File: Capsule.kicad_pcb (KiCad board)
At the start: 2 copper layers, 233.5 x 62.1 mm, 77 parts, among them J1 USB_C_Receptacle_USB2.0, SW1 SW_Push, SW10 SW_Push, SW11 SW_Push, SW12 SW_Push, SW13 SW_Push, SW14 SW_Push, SW15 SW_Push, SW16 SW_Push, SW17 SW_Push, SW18 SW_Push, SW19 SW_Push, SW2 SW_Push, SW20 SW_Push, SW21 SW_Push, SW22 SW_Push, SW23 SW_Push, SW24 SW_Push, SW25 SW_Push, SW26 SW_Push, SW27 SW_Push, SW28 SW_Push, SW29 SW_Push, SW3 SW_Push, SW30 SW_Push, SW4 SW_Push, SW5 SW_Push, SW6 SW_Push, SW7 SW_Push, SW8 SW_Push, SW9 SW_Push, U1 ATmega32U4-A, U2 TPD2S017, Y1 Crystal_GND24

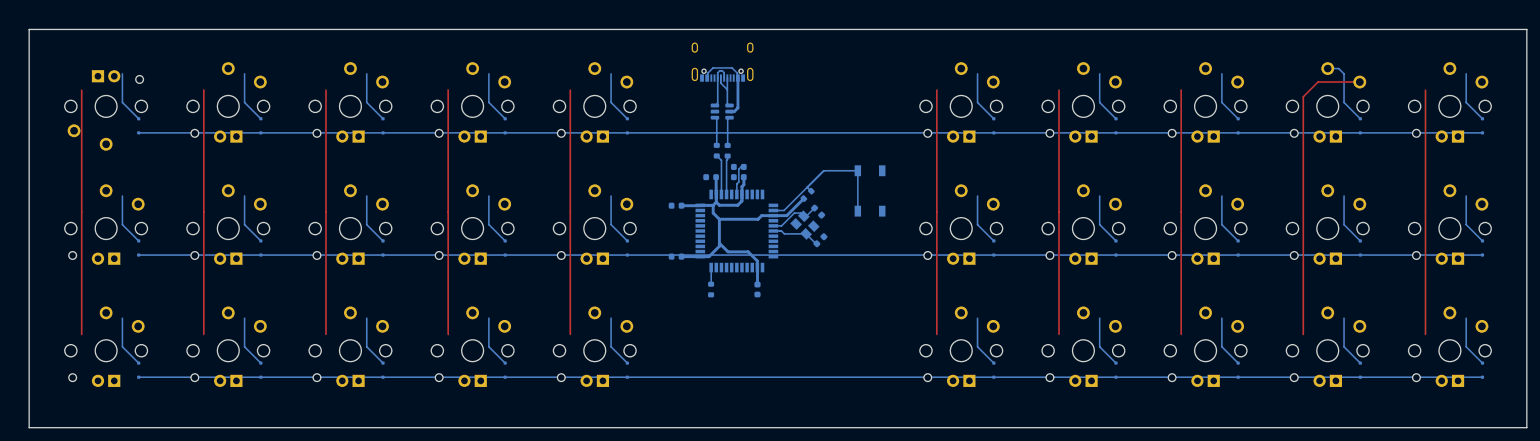
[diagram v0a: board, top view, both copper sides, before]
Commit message: pcb refactor
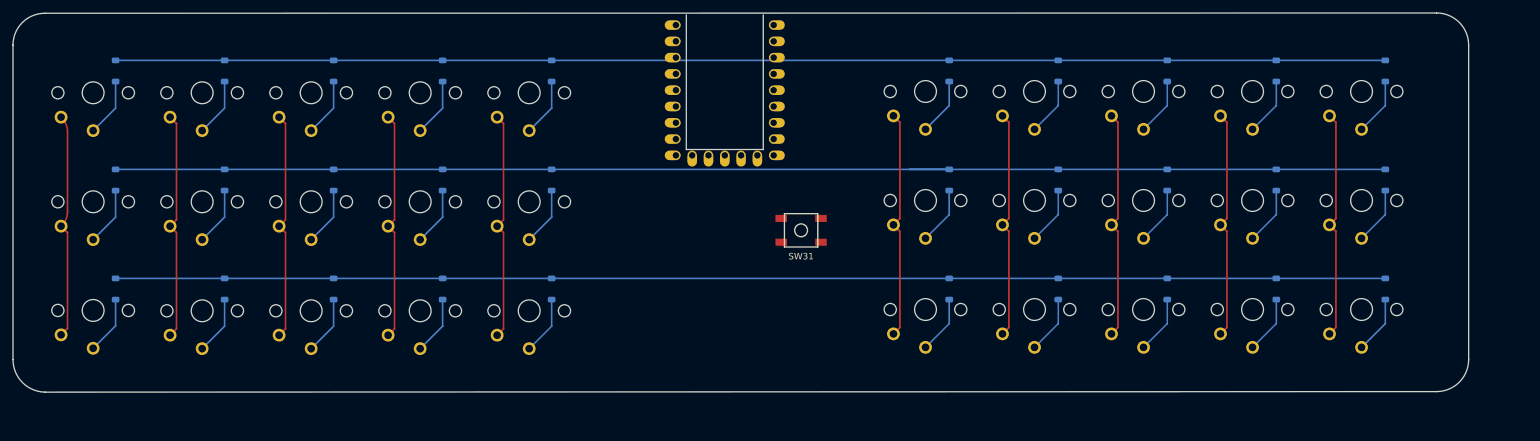
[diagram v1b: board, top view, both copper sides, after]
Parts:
- removed C1, C2: 22p, C_0603_1608Metric
- removed C3, C4, C5, C6: 0.1u, C_0603_1608Metric
- removed C7: 4.7u, C_0603_1608Metric
- removed C8: 1u, C_0603_1608Metric
- removed J1: USB_C_Receptacle_USB2.0, USB_C_Receptacle_XKB_U262-16XN-4BVC11
- removed R1, R2: 22, Resistor_SMD:R_0603_1608Metric
- removed R3, R4: 10k, Resistor_SMD:R_0603_1608Metric
- removed RST: SW_SPST, SW_SPST_TL3342
- removed U2: TPD2S017, SOT-23-6
- removed Y1: Crystal_GND24, Crystal_SMD_3225-4Pin_3.2x2.5mm
- added SW31: SW_Push, random-keyboard-parts:SKQG-1155865, F.Cu at (142.9, 53.9)
- D1, D10, D11, D12, D13, D14, D15, D16, D17, D18, D19, D2, D20, D21, D22, D23, D24, D25, D26, D27, D28, D29, D3, D30, D4, D5, D6, D7, D8, D9: footprint D_SOD-323F -> Diode_SMD:D_SOD-123
- SW1, SW10, SW11, SW12, SW13, SW14, SW15, SW16, SW17, SW18, SW19, SW2, SW20, SW21, SW22, SW23, SW24, SW25, SW26, SW27, SW28, SW29, SW3, SW30, SW4, SW5, SW6, SW7, SW8, SW9: value SW_Push -> SW; footprint Kailh_Choc:KailhChoc-1U -> miketronic_fplib:MB_KailhChoc-1U
- U1: value ATmega32U4-A -> rp2040-zero; footprint TQFP-44_10x10mm_P0.8mm -> mcu:rp2040-zero-tht
- moved U1 22.0 mm to (131.0, 32.0), turned to 180 degrees
- moved D30 19.7 mm to (234.0, 63.0), turned to -90 degrees
- moved D20 18.5 mm to (234.0, 46.0), turned to -90 degrees
- moved D29 18.2 mm to (217.0, 63.0), turned to -90 degrees
- moved D10 17.4 mm to (234.0, 29.0), turned to -90 degrees
- moved D25 17.3 mm to (104.0, 63.0), turned to -90 degrees
- moved D19 16.9 mm to (217.0, 46.0), turned to -90 degrees
- moved D28 16.8 mm to (200.0, 63.0), turned to -90 degrees
- moved D24 16.0 mm to (87.0, 63.0), turned to -90 degrees
- moved D15 15.9 mm to (104.0, 46.0), turned to -90 degrees
- moved D9 15.7 mm to (217.0, 29.0), turned to -90 degrees
- moved D27 15.5 mm to (183.0, 63.0), turned to -90 degrees
- moved D18 15.3 mm to (200.0, 46.0), turned to -90 degrees
- moved SW30 14.9 mm to (229.6, 68.9)
- moved D23 14.8 mm to (70.0, 63.0), turned to -90 degrees
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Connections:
- D1 pad 2: N$1 -> Net-(D1-Pad2)
- D10 pad 2: N$10 -> Net-(D10-Pad2)
- D11 pad 2: N$11 -> Net-(D11-Pad2)
- D12 pad 2: N$12 -> Net-(D12-Pad2)
- D13 pad 2: N$13 -> Net-(D13-Pad2)
- D14 pad 2: N$14 -> Net-(D14-Pad2)
- D15 pad 2: N$15 -> Net-(D15-Pad2)
- D16 pad 2: N$16 -> Net-(D16-Pad2)
- D17 pad 2: N$17 -> Net-(D17-Pad2)
- D18 pad 2: N$18 -> Net-(D18-Pad2)
- D19 pad 2: N$19 -> Net-(D19-Pad2)
- D2 pad 2: N$2 -> Net-(D2-Pad2)
- D20 pad 2: N$20 -> Net-(D20-Pad2)
- D21 pad 2: N$21 -> Net-(D21-Pad2)
- D22 pad 2: N$22 -> Net-(D22-Pad2)
- D23 pad 2: N$23 -> Net-(D23-Pad2)
- D24 pad 2: N$24 -> Net-(D24-Pad2)
- D25 pad 2: N$25 -> Net-(D25-Pad2)
- D26 pad 2: N$26 -> Net-(D26-Pad2)
- D27 pad 2: N$27 -> Net-(D27-Pad2)
- D28 pad 2: N$28 -> Net-(D28-Pad2)
- D29 pad 2: N$29 -> Net-(D29-Pad2)
- D3 pad 2: N$3 -> Net-(D3-Pad2)
- D30 pad 2: N$30 -> Net-(D30-Pad2)
- D4 pad 2: N$4 -> Net-(D4-Pad2)
- D5 pad 2: N$5 -> Net-(D5-Pad2)
- D6 pad 2: N$6 -> Net-(D6-Pad2)
- D7 pad 2: N$7 -> Net-(D7-Pad2)
- D8 pad 2: N$8 -> Net-(D8-Pad2)
- D9 pad 2: N$9 -> Net-(D9-Pad2)
- SW1 pad 1: COL0 -> Net-(D1-Pad2)
- SW1 pad 2: N$1 -> COL0
- SW10 pad 1: COL11 -> Net-(D10-Pad2)
- SW10 pad 2: N$10 -> COL9
- SW11 pad 1: COL0 -> Net-(D11-Pad2)
- SW11 pad 2: N$11 -> COL0
- SW12 pad 1: COL1 -> Net-(D12-Pad2)
- SW12 pad 2: N$12 -> COL1
- SW13 pad 1: COL2 -> Net-(D13-Pad2)
- SW13 pad 2: N$13 -> COL2
- SW14 pad 1: COL3 -> Net-(D14-Pad2)
- SW14 pad 2: N$14 -> COL3
- SW15 pad 1: COL4 -> Net-(D15-Pad2)
- SW15 pad 2: N$15 -> COL4
- SW16 pad 1: COL7 -> Net-(D16-Pad2)
- SW16 pad 2: N$16 -> COL5
- SW17 pad 1: COL8 -> Net-(D17-Pad2)
- SW17 pad 2: N$17 -> COL6
- SW18 pad 1: COL9 -> Net-(D18-Pad2)
- SW18 pad 2: N$18 -> COL7
- SW19 pad 1: COL10 -> Net-(D19-Pad2)
- SW19 pad 2: N$19 -> COL8
- SW2 pad 1: COL1 -> Net-(D2-Pad2)
- SW2 pad 2: N$2 -> COL1
- SW20 pad 1: COL11 -> Net-(D20-Pad2)
- SW20 pad 2: N$20 -> COL9
- SW21 pad 1: COL0 -> Net-(D21-Pad2)
- SW21 pad 2: N$21 -> COL0
- SW22 pad 1: COL1 -> Net-(D22-Pad2)
- SW22 pad 2: N$22 -> COL1
- SW23 pad 1: COL2 -> Net-(D23-Pad2)
- SW23 pad 2: N$23 -> COL2
- SW24 pad 1: COL3 -> Net-(D24-Pad2)
- SW24 pad 2: N$24 -> COL3
- SW25 pad 1: COL4 -> Net-(D25-Pad2)
- SW25 pad 2: N$25 -> COL4
- SW26 pad 1: COL7 -> Net-(D26-Pad2)
- SW26 pad 2: N$26 -> COL5
- SW27 pad 1: COL8 -> Net-(D27-Pad2)
- SW27 pad 2: N$27 -> COL6
- SW28 pad 1: COL9 -> Net-(D28-Pad2)
- SW28 pad 2: N$28 -> COL7
- SW29 pad 1: COL10 -> Net-(D29-Pad2)
- SW29 pad 2: N$29 -> COL8
- SW3 pad 1: COL2 -> Net-(D3-Pad2)
- SW3 pad 2: N$3 -> COL2
- SW30 pad 1: COL11 -> Net-(D30-Pad2)
- SW30 pad 2: N$30 -> COL9
- SW4 pad 1: COL3 -> Net-(D4-Pad2)
- SW4 pad 2: N$4 -> COL3
- SW5 pad 1: COL4 -> Net-(D5-Pad2)
- SW5 pad 2: N$5 -> COL4
- SW6 pad 1: COL7 -> Net-(D6-Pad2)
- SW6 pad 2: N$6 -> COL5
- SW7 pad 1: COL8 -> Net-(D7-Pad2)
- SW7 pad 2: N$7 -> COL6
- SW8 pad 1: COL9 -> Net-(D8-Pad2)
- SW8 pad 2: N$8 -> COL7
- SW9 pad 1: COL10 -> Net-(D9-Pad2)
- SW9 pad 2: N$9 -> COL8
- U1 pad 1: (no net) -> unconnected-(U1-0-Pad1)
- U1 pad 10: ROW2 -> unconnected-(U1-9-Pad10)
- U1 pad 11: COL0 -> unconnected-(U1-10-Pad11)
- U1 pad 12: COL4 -> unconnected-(U1-11-Pad12)
- U1 pad 13: mcu/~{RESET} -> unconnected-(U1-12-Pad13)
- U1 pad 14: VCC -> unconnected-(U1-13-Pad14)
- U1 pad 15: GND -> unconnected-(U1-14-Pad15)
- U1 pad 16: mcu/XTAL2 -> unconnected-(U1-15-Pad16)
- U1 pad 17: mcu/XTAL1 -> unconnected-(U1-26-Pad17)
- U1 pad 18: COL9 -> unconnected-(U1-27-Pad18)
- U1 pad 19: COL10 -> unconnected-(U1-28-Pad19)
- U1 pad 2: VCC -> unconnected-(U1-1-Pad2)
- U1 pad 20: COL11 -> unconnected-(U1-29-Pad20)
- U1 pad 21: (no net) -> unconnected-(U1-3V3-Pad21)
- U1 pad 22: (no net) -> unconnected-(U1-GND-Pad22)
- U1 pad 23: GND -> unconnected-(U1-5V-Pad23)
- U1 pad 3: mcu/D- -> unconnected-(U1-2-Pad3)
- U1 pad 4: mcu/D+ -> unconnected-(U1-3-Pad4)
- U1 pad 5: GND -> unconnected-(U1-4-Pad5)
- U1 pad 6: mcu/UCAP -> unconnected-(U1-5-Pad6)
- U1 pad 7: VCC -> unconnected-(U1-6-Pad7)
- U1 pad 8: ROW0 -> unconnected-(U1-7-Pad8)
- U1 pad 9: ROW1 -> unconnected-(U1-8-Pad9)
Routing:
- net (no net): track 495.3 -> 0.00 mm
- net ROW1: track 0.00 -> 204.2 mm
- net ROW0: track 0.00 -> 198.0 mm
- net VCC: track 69.1 -> 0.00 mm
- net COL10: track 46.8 -> 0.00 mm
- net COL11: track 38.1 -> 0.00 mm
- net COL5: track 0.00 -> 35.7 mm
- net COL1: track 0.00 -> 35.7 mm
- net COL6: track 0.00 -> 35.7 mm
- net COL0: track 0.00 -> 35.6 mm
- net mcu/~{RESET}: track 26.5 -> 0.00 mm
- net ROW2: track 209.6 -> 198.0 mm
- net N$9: track 10.9 -> 0.00 mm
- net Net-(D5-Pad2): track 0.00 -> 9.10 mm
- net Net-(D4-Pad2): track 0.00 -> 9.10 mm
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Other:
- board size 233.5 x 62.1 mm -> 227 x 59.1 mm

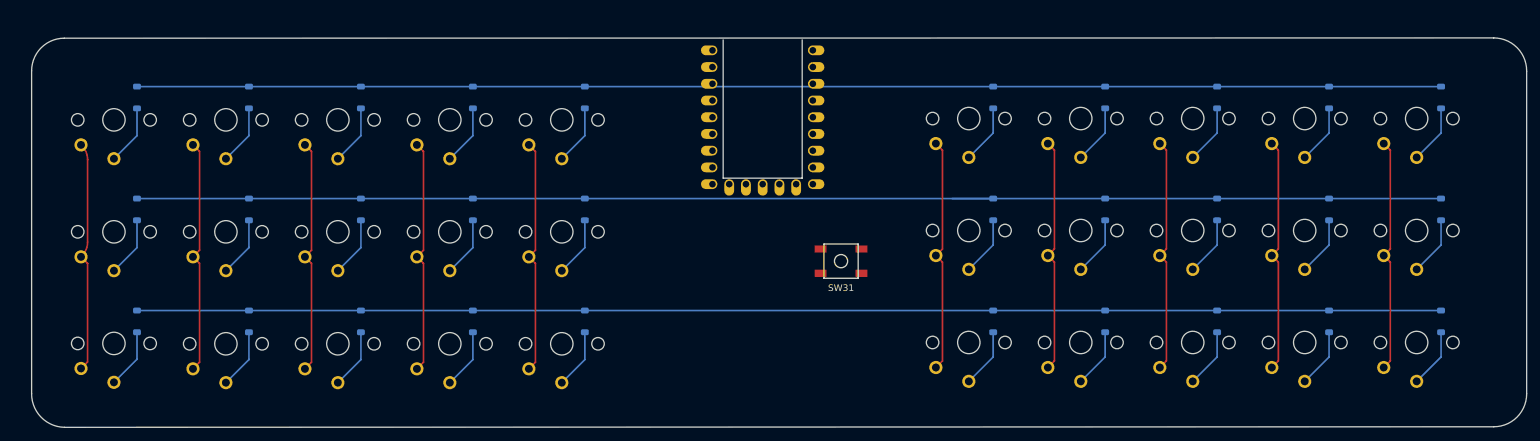
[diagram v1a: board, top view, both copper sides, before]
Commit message: add submodules
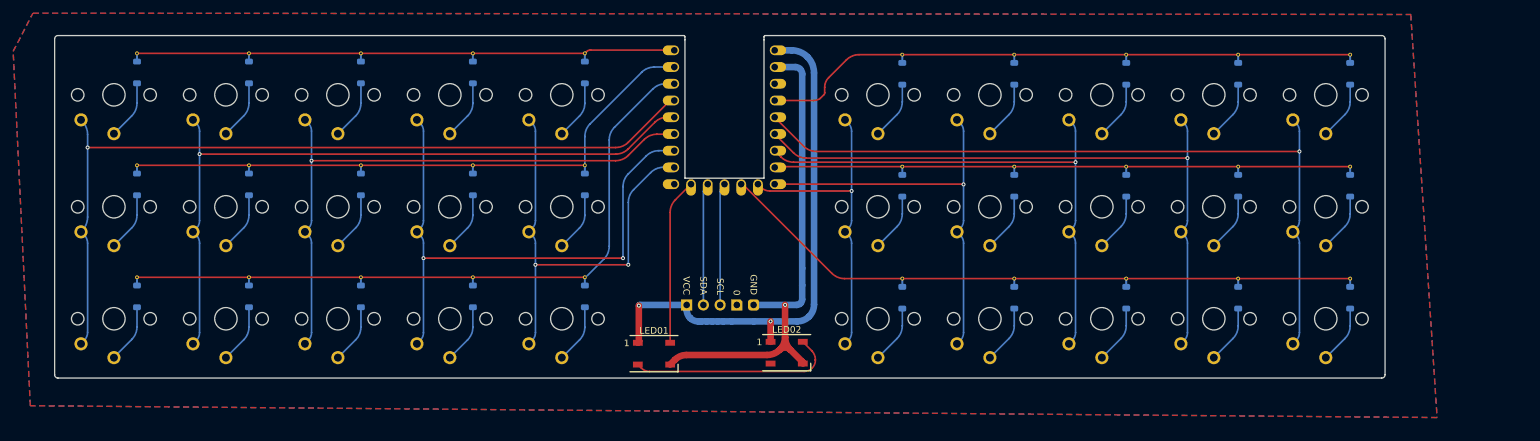
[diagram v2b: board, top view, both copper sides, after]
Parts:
- removed SW31: SW_Push, random-keyboard-parts:SKQG-1155865
- added Connector1: MB_i2c_header, miketronic_fplib:MB_I2C_Breakout_reverse, F.Cu at (129.6, 60.5)
- added LED01: WS2812B, LED_SMD:LED_WS2812B_PLCC4_5.0x5.0mm_P3.2mm, F.Cu at (114.5, 67.9)
- added LED02: WS2812B, LED_SMD:LED_WS2812B_PLCC4_5.0x5.0mm_P3.2mm, F.Cu at (134.7, 67.8)
- D1, D10, D11, D12, D13, D14, D15, D16, D17, D18, D19, D2, D20, D21, D22, D23, D24, D25, D26, D27, D28, D29, D3, D30, D4, D5, D6, D7, D8, D9: footprint Diode_SMD:D_SOD-123 -> miketronic_fplib:MB_D_SOD-123_1PAD
- SW1, SW10, SW11, SW12, SW13, SW14, SW15, SW16, SW17, SW18, SW19, SW2, SW20, SW21, SW22, SW23, SW24, SW25, SW26, SW27, SW28, SW29, SW3, SW30, SW4, SW5, SW6, SW7, SW8, SW9: footprint miketronic_fplib:MB_KailhChoc-1U -> miketronic_fplib:MB_KailhChoc-1U_17mm
- U1: footprint mcu:rp2040-zero-tht -> miketronic_fplib:MB_rp2040-zero-tht
- moved D10 14.3 mm to (220.2, 25.4)
- moved D16 14.3 mm to (152.2, 42.4)
- moved D17 14.3 mm to (169.2, 42.4)
- moved D18 14.3 mm to (186.2, 42.4)
- moved D19 14.3 mm to (203.2, 42.4)
- moved D20 14.3 mm to (220.2, 42.4)
- moved D26 14.3 mm to (152.2, 59.4)
- moved D27 14.3 mm to (169.2, 59.4)
- moved D28 14.3 mm to (186.2, 59.4)
- moved D29 14.3 mm to (203.2, 59.4)
- moved D30 14.3 mm to (220.2, 59.4)
- moved D6 14.3 mm to (152.2, 25.4)
- moved D7 14.3 mm to (169.2, 25.4)
- moved D8 14.3 mm to (186.2, 25.4)
- moved D9 14.3 mm to (203.2, 25.4)
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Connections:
- D10 pad 1: ROW0 -> ROW3
- D16 pad 1: ROW1 -> ROW4
- D17 pad 1: ROW1 -> ROW4
- D18 pad 1: ROW1 -> ROW4
- D19 pad 1: ROW1 -> ROW4
- D20 pad 1: ROW1 -> ROW4
- D26 pad 1: ROW2 -> ROW5
- D27 pad 1: ROW2 -> ROW5
- D28 pad 1: ROW2 -> ROW5
- D29 pad 1: ROW2 -> ROW5
- D30 pad 1: ROW2 -> ROW5
- D6 pad 1: ROW0 -> ROW3
- D7 pad 1: ROW0 -> ROW3
- D8 pad 1: ROW0 -> ROW3
- D9 pad 1: ROW0 -> ROW3
- U1 pad 1: unconnected-(U1-0-Pad1) -> ROW0
- U1 pad 10: unconnected-(U1-9-Pad10) -> RGB
- U1 pad 11: unconnected-(U1-10-Pad11) -> SDA
- U1 pad 12: unconnected-(U1-11-Pad12) -> SCL
- U1 pad 13: unconnected-(U1-12-Pad13) -> ROW5
- U1 pad 14: unconnected-(U1-13-Pad14) -> COL5
- U1 pad 15: unconnected-(U1-14-Pad15) -> COL6
- U1 pad 16: unconnected-(U1-15-Pad16) -> ROW4
- U1 pad 17: unconnected-(U1-26-Pad17) -> COL7
- U1 pad 18: unconnected-(U1-27-Pad18) -> COL8
- U1 pad 19: unconnected-(U1-28-Pad19) -> COL9
- U1 pad 2: unconnected-(U1-1-Pad2) -> ROW1
- U1 pad 20: unconnected-(U1-29-Pad20) -> ROW3
- U1 pad 22: unconnected-(U1-GND-Pad22) -> GND
- U1 pad 23: unconnected-(U1-5V-Pad23) -> VCC
- U1 pad 3: unconnected-(U1-2-Pad3) -> ROW2
- U1 pad 4: unconnected-(U1-3-Pad4) -> COL0
- U1 pad 5: unconnected-(U1-4-Pad5) -> COL1
- U1 pad 6: unconnected-(U1-5-Pad6) -> COL2
- U1 pad 7: unconnected-(U1-6-Pad7) -> COL3
- U1 pad 8: unconnected-(U1-7-Pad8) -> COL4
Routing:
- net ROW0: track 198.0 -> 81.8 mm
- net ROW1: track 204.2 -> 92.0 mm
- net ROW5: track 0.00 -> 98.3 mm
- net ROW2: track 198.0 -> 103.8 mm
- net ROW3: track 0.00 -> 91.1 mm
- net COL0: track 35.6 -> 126.5 mm, vias 0 -> 1
- net ROW4: track 0.00 -> 87.2 mm
- net VCC: track 0.00 -> 82.1 mm, vias 0 -> 2
- net COL9: track 35.7 -> 116.7 mm, vias 0 -> 1
- net GND: track 0.00 -> 77.9 mm, vias 0 -> 1
- net COL1: track 35.7 -> 109.1 mm, vias 0 -> 1
- net COL8: track 35.7 -> 99.1 mm, vias 0 -> 1
- net COL2: track 35.7 -> 91.5 mm, vias 0 -> 1
- net COL3: track 35.7 -> 86.6 mm, vias 0 -> 2
- net COL7: track 35.7 -> 81.2 mm, vias 0 -> 1
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- added copper zone on B.Cu, net GND
- added copper zone on F.Cu, net GND
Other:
- board size 227 x 59.1 mm -> 202 x 52 mm
- board text added: "Capsule v1.0 github.com/miketronic"
